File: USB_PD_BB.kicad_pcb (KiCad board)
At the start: 2 copper layers, 70 x 50 mm, 7 parts, among them CN1 53375-0410, CN2 10126-5212PC, CN3 UJC-HP-3-SMT-TR, U3 IP2721D

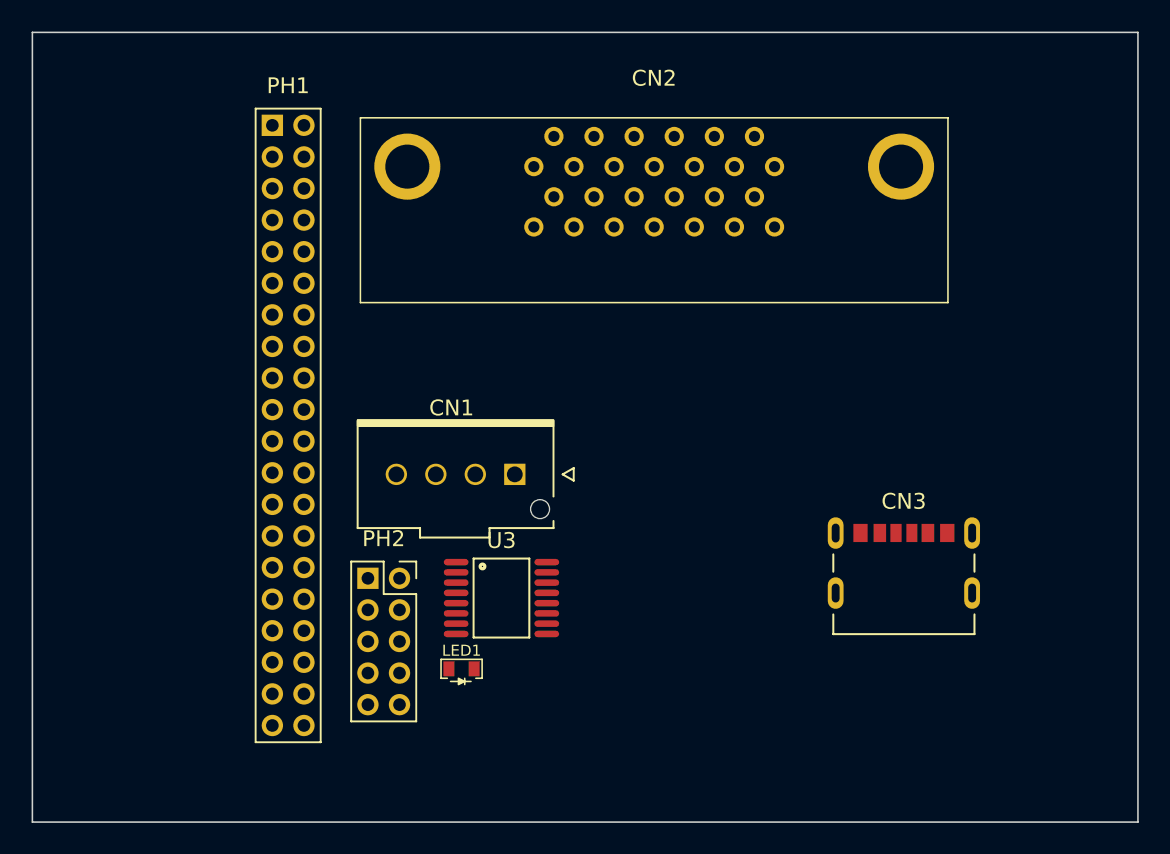
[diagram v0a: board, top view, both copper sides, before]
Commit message: add FET ans Switch
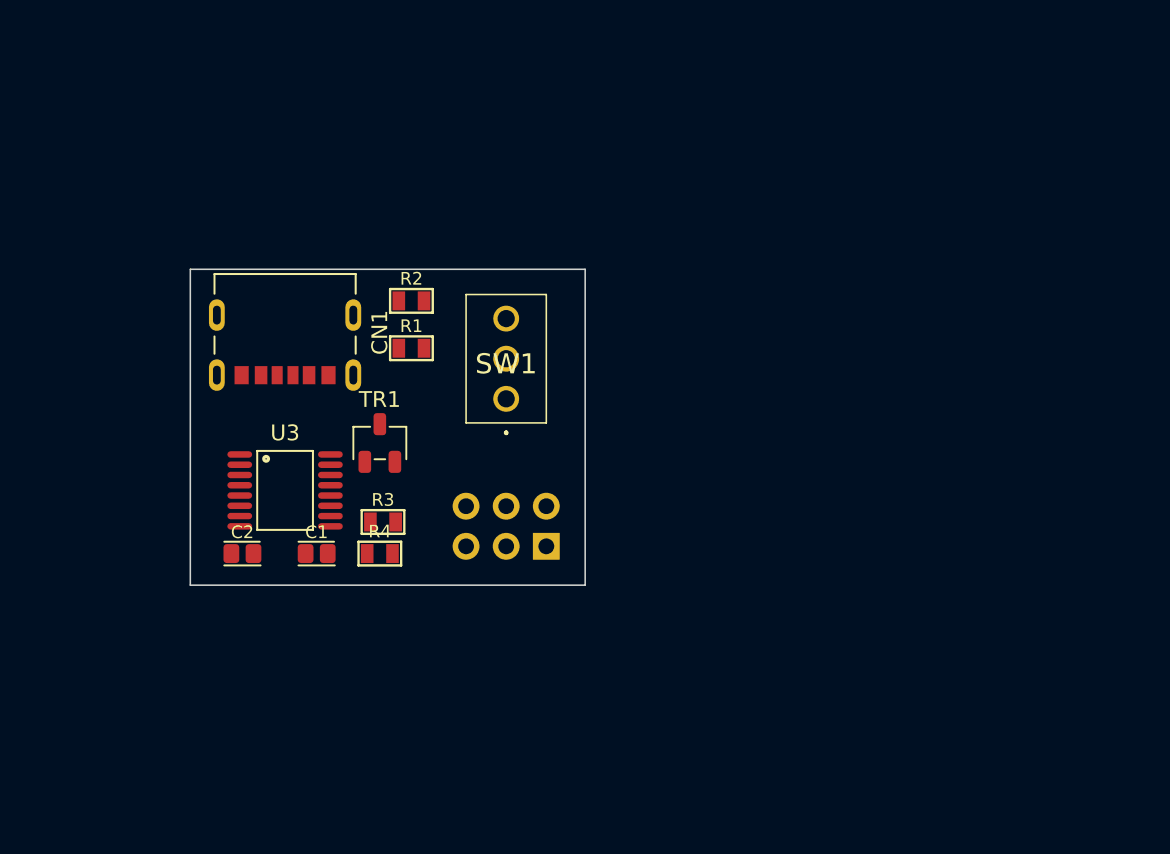
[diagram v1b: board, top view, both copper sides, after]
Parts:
- removed CN2: 10126-5212PC, Connector:10126-5212PC
- removed CN3: UJC-HP-3-SMT-TR, Connector:UJC-HP-3-SMT-TR
- removed LED1: Value, Basic:LED1608mRED
- removed PH2: PinSocket2mm_2x5, PinSocket:PinSocket2mm_2x5
- added C1: 1uF/50V, Basic:CAP1608m, F.Cu at (118.0, 98.0)
- added C2: Value, Basic:CAP1608m, F.Cu at (113.3, 98.0)
- added R1: 5.1k, Basic:REG1608m, F.Cu at (124.0, 85.0)
- added R2: 5.1k, Basic:REG1608m, F.Cu at (124.0, 82.0)
- added R3: 100k, Basic:REG1608m, F.Cu at (122.2, 96.0)
- added R4: 100k, Basic:REG1608m, F.Cu at (122.0, 98.0)
- added SW1: 2MS1-T1-B4-VS2-S-E, Switch:2MS1-T1-B4-VS2-Q-E-S, F.Cu at (130.0, 88.2)
- added TR1: AO3400A, Discrete:AO3400A, F.Cu at (122.0, 91.0)
- CN1: value 53375-0410 -> UJC-HP-3-SMT-TR; footprint Connector:53375-0410 -> Connector:UJC-HP-3-SMT-TR
- PH1: value PinSocket2mm_2x20 -> PinHeader3x2; footprint PinSocket:PinSocket2mm_2x20 -> PinHeader:PinHeader3x2; moved to B.Cu
- moved PH1 30.8 mm to (132.5, 97.5), turned to 90 degrees
- moved U3 15.3 mm to (116.0, 94.0)
- moved CN1 12.5 mm to (116.0, 86.7), turned to 180 degrees
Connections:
- U3 pad 1: unconnected-(U3-VBUSG-Pad1) -> Net-(U3-VBUSG)
- U3 pad 11: unconnected-(U3-SEL-Pad11) -> /SEL
- U3 pad 12: unconnected-(U3-CC2-Pad12) -> /CC2
- U3 pad 13: unconnected-(U3-CC1-Pad13) -> /CC1
- U3 pad 16: unconnected-(U3-VBUS-Pad16) -> /Vout
- U3 pad 2: unconnected-(U3-VIN-Pad2) -> Vin
- U3 pad 5: unconnected-(U3-GND-Pad5) -> GND
- U3 pad 6: unconnected-(U3-SELP-Pad6) -> /SELP
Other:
- board size 70 x 50 mm -> 25 x 20 mm

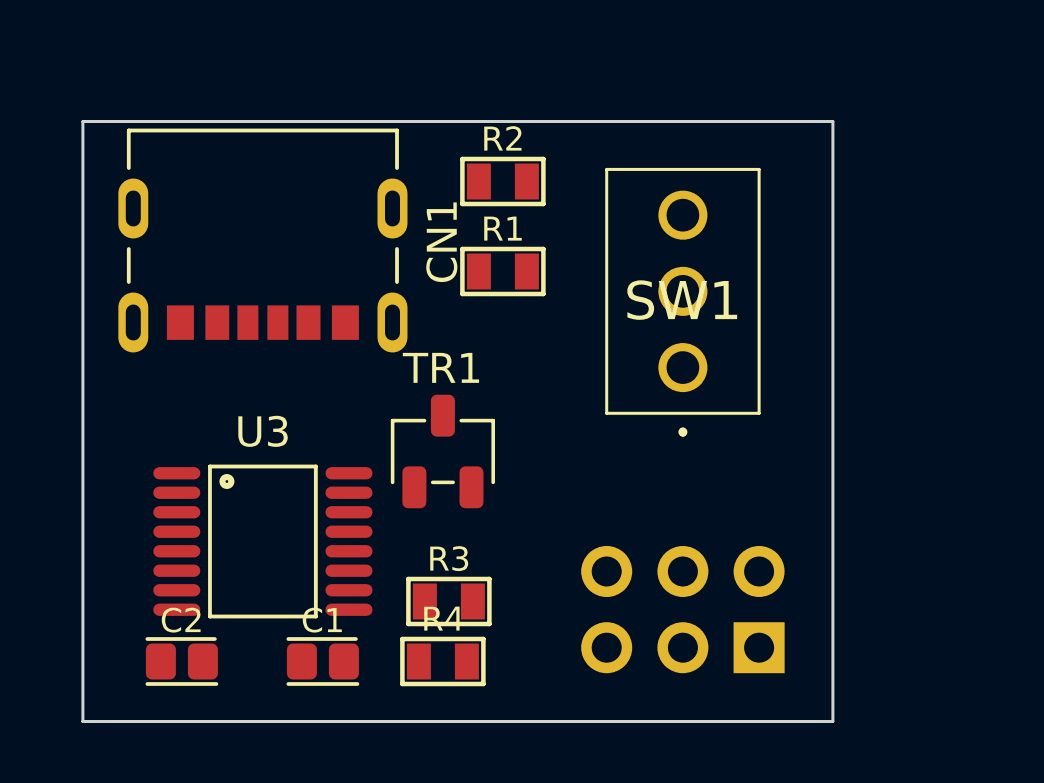
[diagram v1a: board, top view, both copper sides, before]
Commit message: rough artwork.
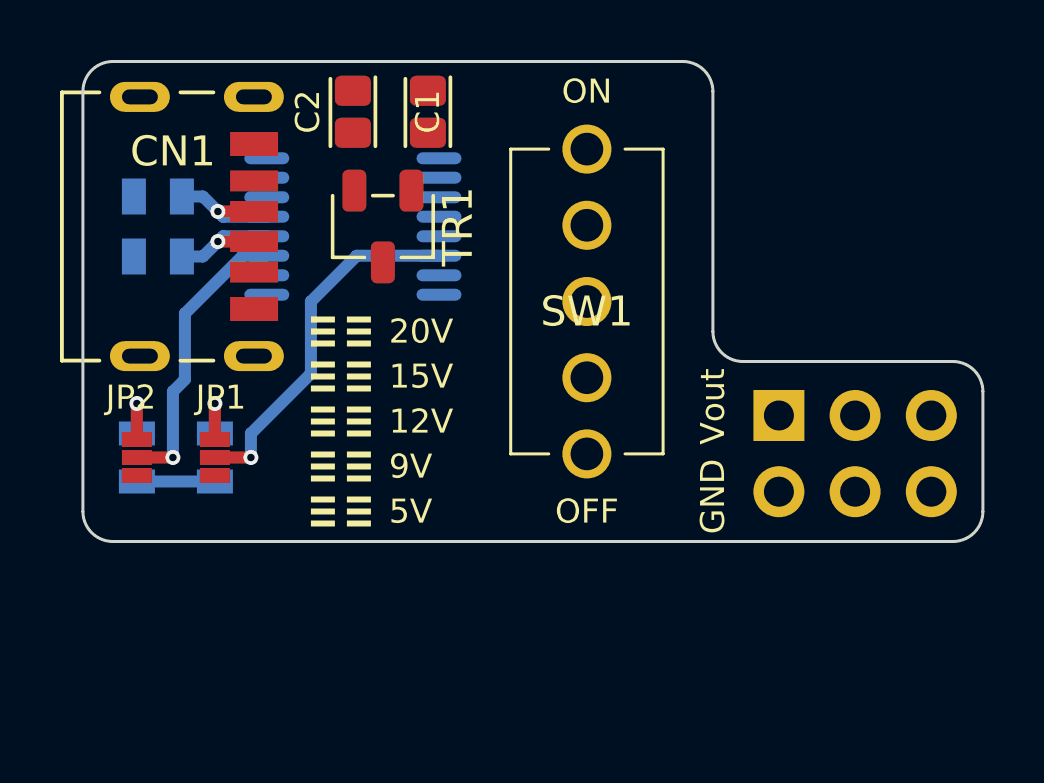
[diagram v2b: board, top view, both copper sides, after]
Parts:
- added JP1: ~, Jumper:SolderJumperSel, F.Cu at (114.4, 91.2)
- added JP2: ~, Jumper:SolderJumperSel, F.Cu at (111.8, 91.2)
- R1, R2, R3, R4, U3: moved to B.Cu
- moved C2 19.2 mm to (119.0, 79.7), turned to 90 degrees
- moved C1 18.7 mm to (121.5, 79.7), turned to 90 degrees
- moved R1 11.8 mm to (112.5, 82.5), turned to 180 degrees
- moved R2 11.8 mm to (112.5, 84.5), turned to 180 degrees
- moved R3 11.5 mm to (111.8, 91.2), turned to 90 degrees
- moved U3 10.9 mm to (119.0, 83.5), turned to 180 degrees
- moved R4 10.2 mm to (114.4, 91.2), turned to 90 degrees
- moved PH1 7.77 mm to (133.2, 89.8), turned to -90 degrees
- moved TR1 7.76 mm to (120.0, 83.5), turned to 180 degrees
- moved SW1 3.88 mm to (126.8, 86.0)
- moved CN1 3.21 mm to (115.7, 83.5), turned to -90 degrees
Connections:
- PH1 pad 1: unconnected-(PH1-Pad1) -> Net-(PH1-Pad1)
- PH1 pad 2: unconnected-(PH1-Pad2) -> GND
- PH1 pad 3: unconnected-(PH1-Pad3) -> Net-(PH1-Pad1)
- PH1 pad 4: unconnected-(PH1-Pad4) -> GND
- PH1 pad 5: unconnected-(PH1-Pad5) -> Net-(PH1-Pad1)
- PH1 pad 6: unconnected-(PH1-Pad6) -> GND
- R3 pad 2: /SEL -> Net-(JP2-Pad2)
- R4 pad 2: /SELP -> Net-(JP1-Pad2)
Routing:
- net /SELP: track 0.00 -> 12.1 mm, vias 0 -> 1
- net /SEL: track 0.00 -> 9.69 mm, vias 0 -> 1
- net /CC2: track 0.00 -> 4.31 mm, vias 0 -> 1
- net /CC1: track 0.00 -> 4.31 mm, vias 0 -> 1
- net Vin: track 0.00 -> 2.60 mm
- net Net-(JP2-Pad2): track 0.00 -> 2.20 mm, vias 0 -> 1
- net Net-(JP1-Pad2): track 0.00 -> 2.20 mm, vias 0 -> 1
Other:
- board size 25 x 20 mm -> 30 x 16 mm
- board text added: "12V"
- board text added: "15V"
- board text added: "20V"
- board text added: "5V"
- board text added: "9V"
- board text added: "GND"
- board text added: "OFF"
- board text added: "ON"
- board text added: "Vout"
